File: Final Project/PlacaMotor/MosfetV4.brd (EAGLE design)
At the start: 42.2 x 37.3 mm, 15 parts, among them IC1 ATTINY44-SSU

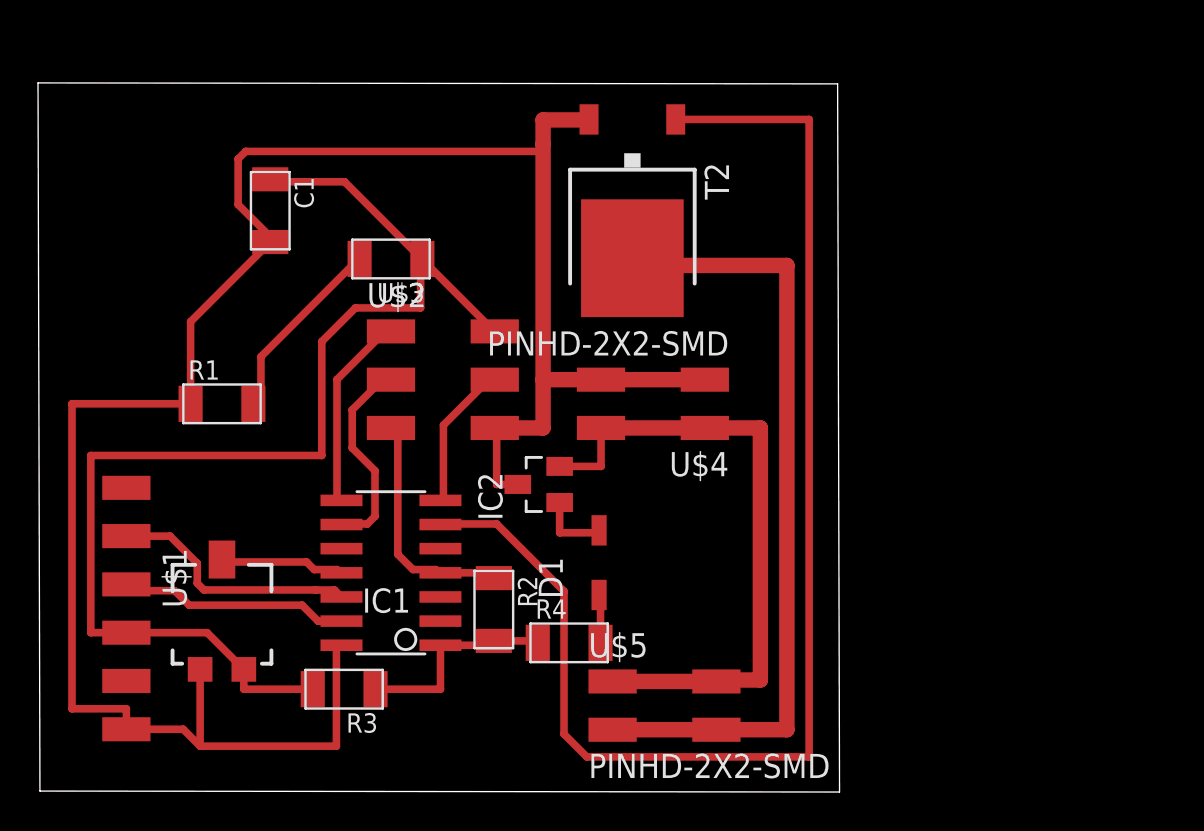
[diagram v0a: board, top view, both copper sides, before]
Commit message: Placa Final plz
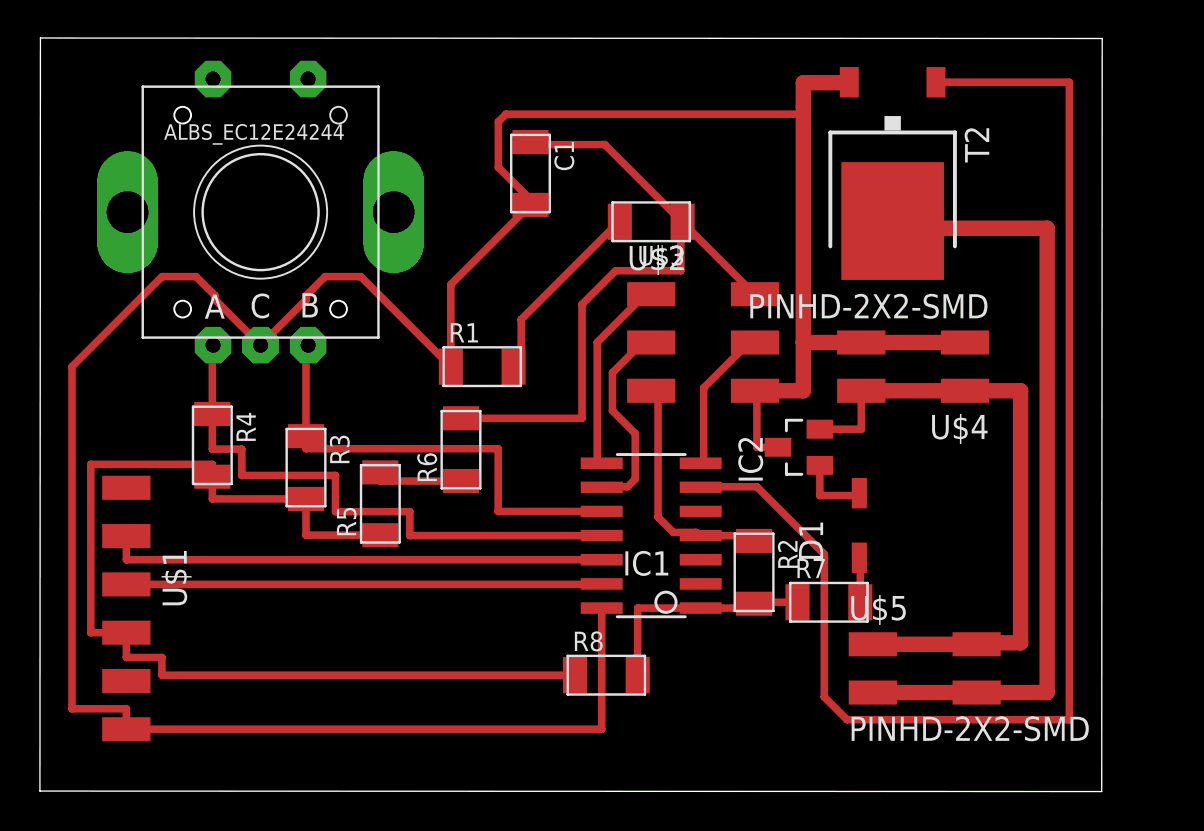
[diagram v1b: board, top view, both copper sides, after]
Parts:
- removed VR1: 5k, SparkFun-Resistors:TRIMPOT-SMD-5MM
- added R5, R6, R7, R8: 0, fab:R1206FAB
- added U$6: ALBS_ENCODER_STEC12E08, Rotary Encoder:STEC12E08
- R3, R4: value 0 -> 10k
- moved R4 21.5 mm to (9.45, 18.0), turned to 270 degrees
- moved IC2 13.8 mm to (40.3, 17.9)
- moved R1 13.8 mm to (23.6, 22.2)
- moved C1 13.8 mm to (26.2, 32.3)
- moved D1 13.8 mm to (43.5, 13.8)
- moved R2 13.8 mm to (37.9, 11.4)
- moved T2 13.8 mm to (45.2, 32.3)
- moved IC1 13.8 mm to (32.5, 13.3)
- moved U$2 13.8 mm to (35.1, 23.4)
- moved U$3 13.8 mm to (32.5, 29.8)
- moved U$4 13.8 mm to (46.5, 22.2)
- moved U$5 13.8 mm to (46.7, 6.30)
- moved R3 11.8 mm to (14.4, 16.9), turned to 270 degrees
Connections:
- removed net ANALOG: IC1.11, VR1.B
- removed net N$12: IC1.10
- new net ENC1: IC1.10, R3.1, U$6.P$B
- new net ENC2: IC1.11, R4.1, U$6.P$A
- net 0: now also U$6.P$C; no longer VR1.C
- net VCC: now also R5.1, R5.2, R6.1, R6.2, R7.1, R7.2, R8.1, R8.2; no longer R3.1, R4.1, VR1.A
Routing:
- net VCC: track 79.0 -> 111.5 mm
- net 0: track 114.4 -> 146.4 mm
- net ENC2: track 0.00 -> 30.5 mm
- net ENC1: track 0.00 -> 24.4 mm
- net RX: track 13.3 -> 26.3 mm
- net TX: track 12.1 -> 25.1 mm
- net ANALOG: track 6.59 -> 0.00 mm
- net MOSFET: track 43.7 -> 42.0 mm
- net 12V: track 34.5 -> 33.9 mm
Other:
- board size 42.2 x 37.3 mm -> 55.9 x 39.6 mm
